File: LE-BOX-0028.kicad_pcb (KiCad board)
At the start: 2 copper layers, 76 x 96 mm, 66 parts, among them P1 MYSX_1.5, P2 CONN_02X03, P3 CONN_01X03, P4 CONN_01X03, Q1 DMP3056L-7, Q2 DMP3056L-7, U1 LD1117DT33TR, U2 TPS61097A, U3 ATSHA204A, U4 RFM69HW, U5 NRF24L01, U6 AT25DF512C, U7 ArduinoProMini, U8 Si7021, U9 TPS61221

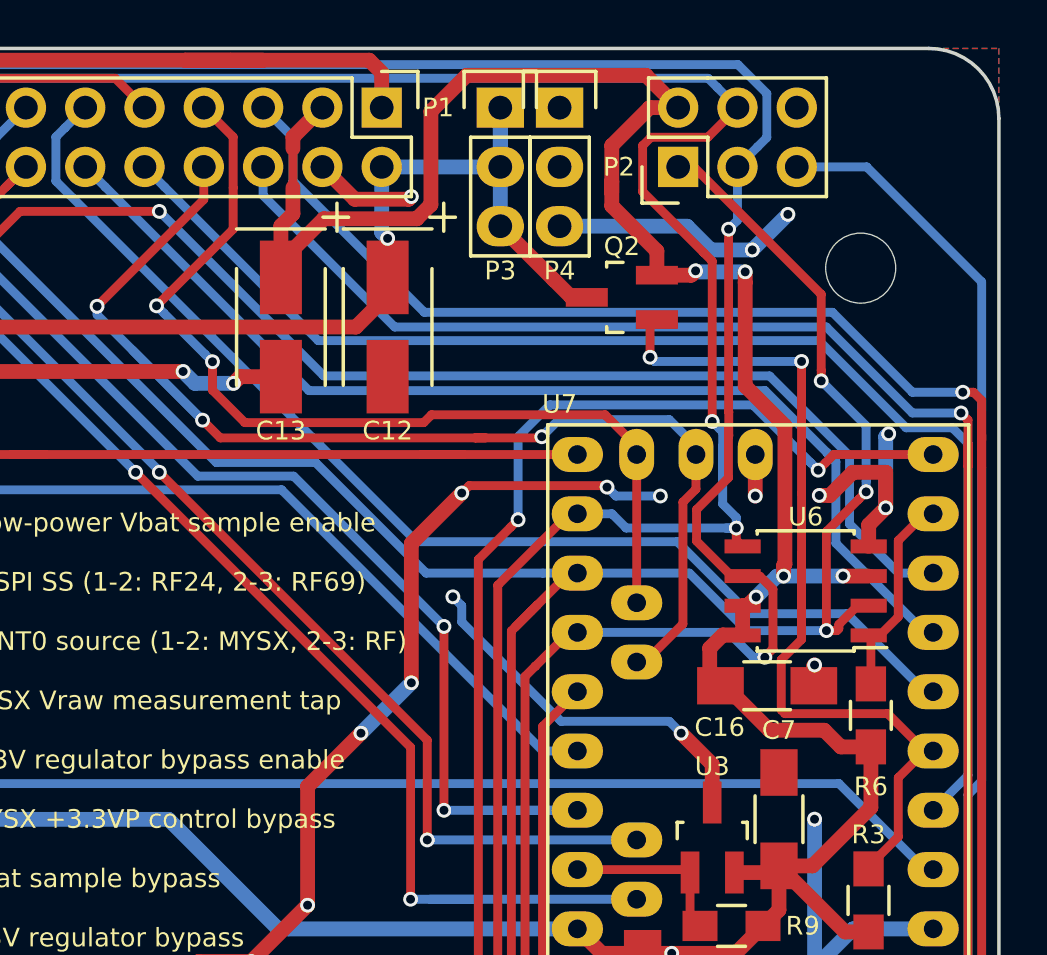
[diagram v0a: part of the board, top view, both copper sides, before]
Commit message: Minor layout beautifications
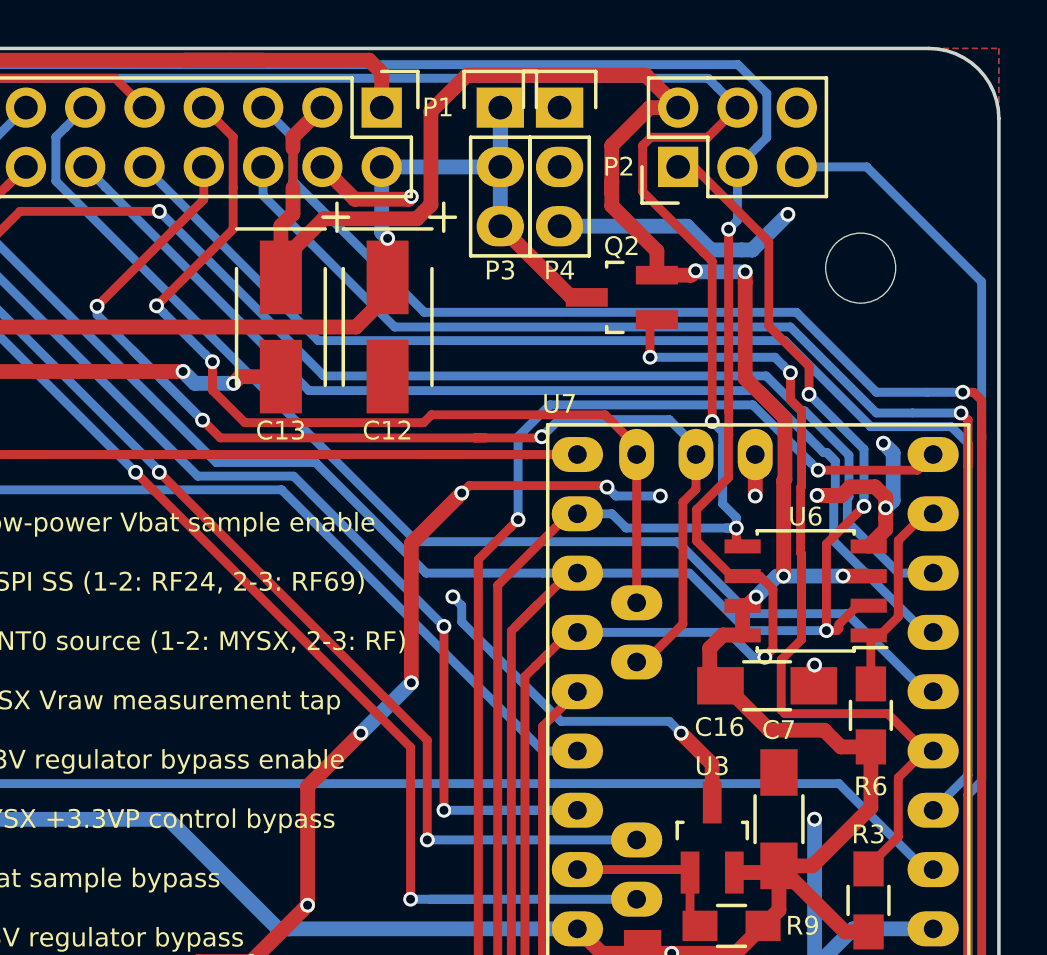
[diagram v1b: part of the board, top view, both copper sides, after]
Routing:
- net GND: track 718.6 -> 717.4 mm, vias 459 -> 458
- net MYSX_3.3V_EN: track 40.5 -> 39.9 mm
